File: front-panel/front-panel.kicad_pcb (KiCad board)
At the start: 2 copper layers, 87 x 326.5 mm, 21 parts

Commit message: Updated panels based on dxf drawings from mech, need to move all holes up 5mm
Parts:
- moved Buck2 11.1 mm to (178.7, 39.2)
- moved H2 6.49 mm to (112.1, 124.3)
- moved H4 6.49 mm to (188.3, 124.3)
- moved H10 4.26 mm to (121.1, 37.0)
- moved H12 4.25 mm to (153.2, 15.7)
- moved H11 4.24 mm to (153.3, 36.9)
- moved H9 4.21 mm to (121.1, 15.8)
- moved SC7 3.75 mm to (108.2, 81.1)
- moved SC14 0.58 mm to (134.1, 67.1)
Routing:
- net Net-(SC14--): track 73.9 -> 16.2 mm
- net Net-(Buck2-BCR+): track 8.04 -> 40.0 mm, vias 0 -> 1
- net Net-(Buck2-BCR-): track 281.3 -> 273.6 mm
- added copper zone on B.Cu, net Net-(Buck2-BCR+)
- added copper zone on B.Cu, net Net-(Buck2-BCR-)
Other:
- outline, holes or cut-outs redrawn

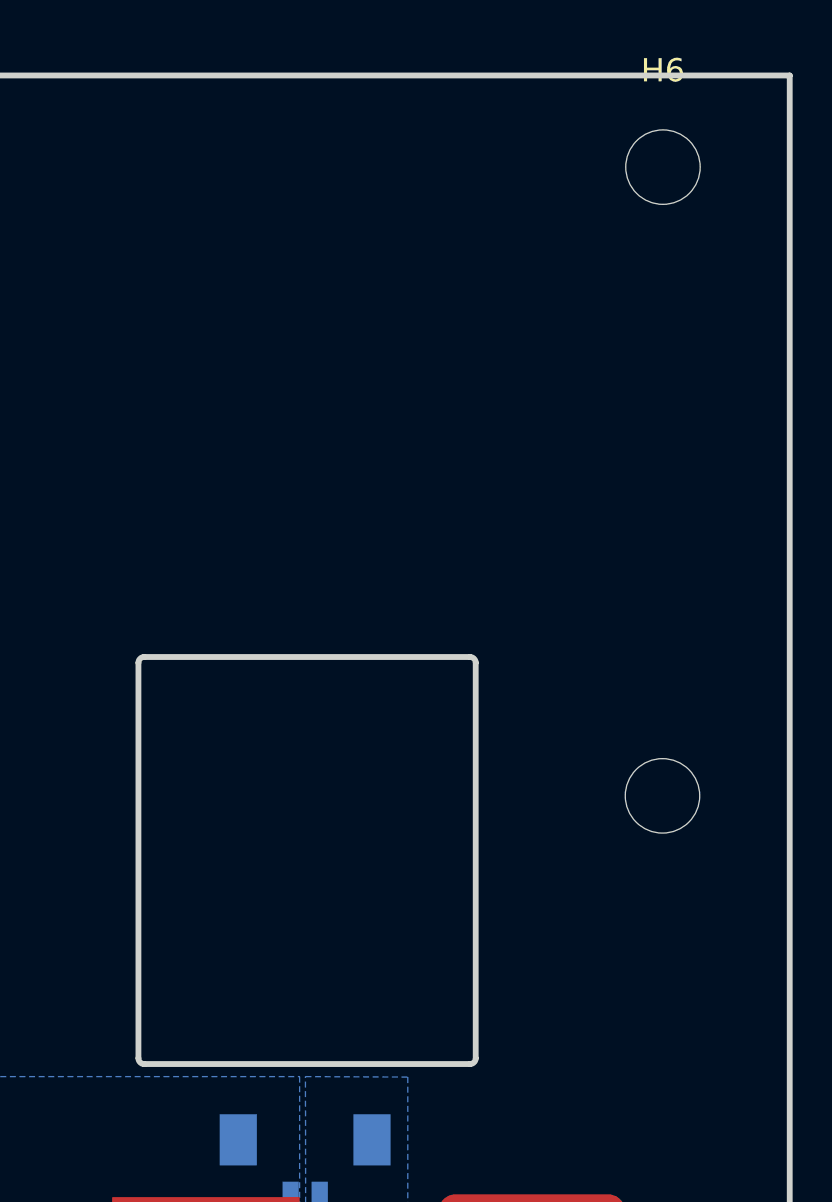
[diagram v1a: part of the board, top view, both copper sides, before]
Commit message: changed ALOT of things, got it to a point to send mech models,solar panel harness on BS need changed
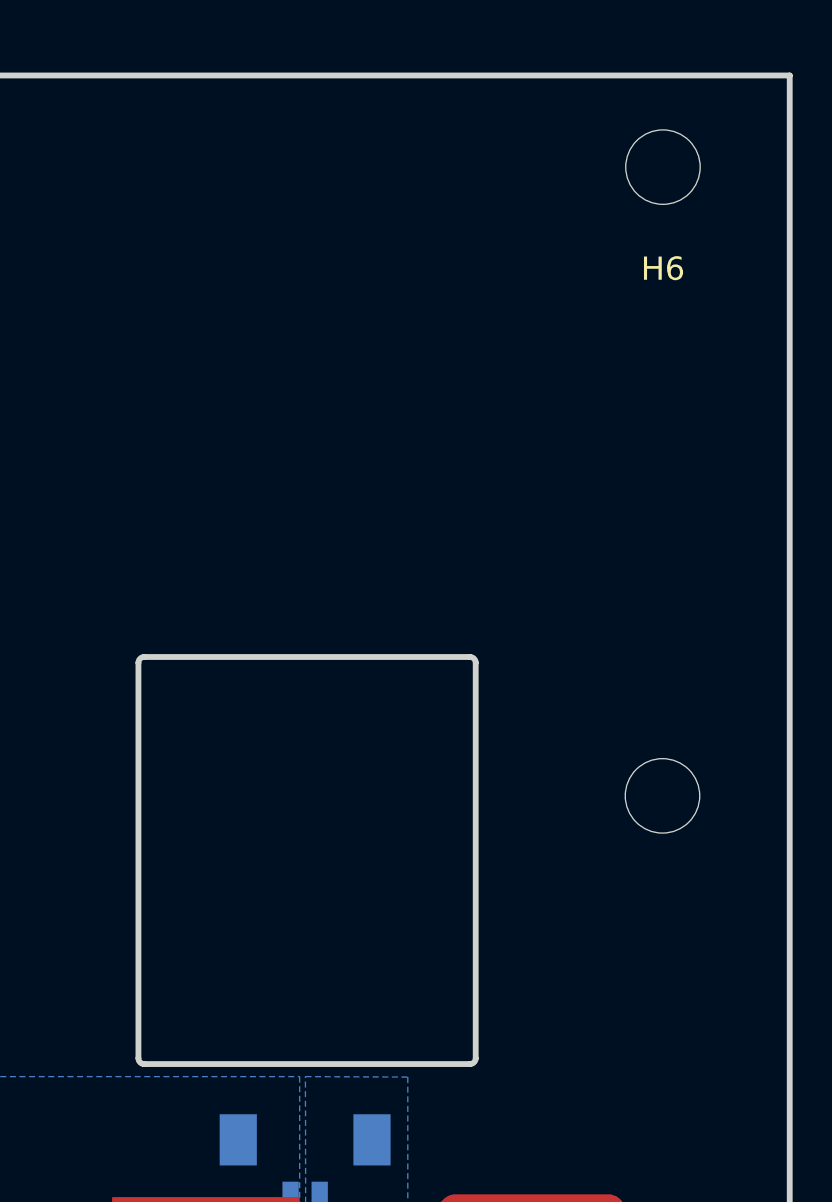
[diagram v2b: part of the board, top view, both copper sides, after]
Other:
- outline, holes or cut-outs redrawn
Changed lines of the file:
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@@
 		(tags "mountinghole M3")
 		(property "Reference" "H6"
-			(at 0 -4.15 0)
+			(at 0 4.38 0)
 			(layer "F.SilkS")
 			(effects
@@
 	)
 	(gr_line
-		(start 179.930046 9.33)
-		(end 165.93 9.33)
-		(stroke
-			(width 0.25)
-			(type default)
-		)
-		(locked yes)
-		(layer "Edge.Cuts")
-	)
-	(gr_rect
-		(start 165.753213 9.403176)
-		(end 180.106766 26.756747)
-		(stroke
-			(width 0.05)
-			(type default)
-		)
-		(fill no)
+		(start 179.930046 9.330001)
+		(end 165.9299 9.33)
+		(stroke
+			(width 0.25)
+			(type default)
+		)
 		(locked yes)
 		(layer "Edge.Cuts")
@@
 		(stroke
 			(width 0.25)
-			(type default)
-		)
-		(locked yes)
+			(type solid)
+		)
+		(locked yes)
